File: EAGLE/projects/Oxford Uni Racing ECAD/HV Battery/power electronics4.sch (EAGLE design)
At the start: 57 parts, among them IC1 4043N, IC2 4001N, IC3 LM555CN, IC4 4071N, IC5 4081N, IC6 4011N, IC7 4011N, K1 T9AS1D12-48=T9A, K2 T9AS5D12-12=T9A, K4 T9AS1D12-48=T9A, K5 T9AS1D12-48=T9A, Q1 BS170, Q2 BS170, Q3 BS170

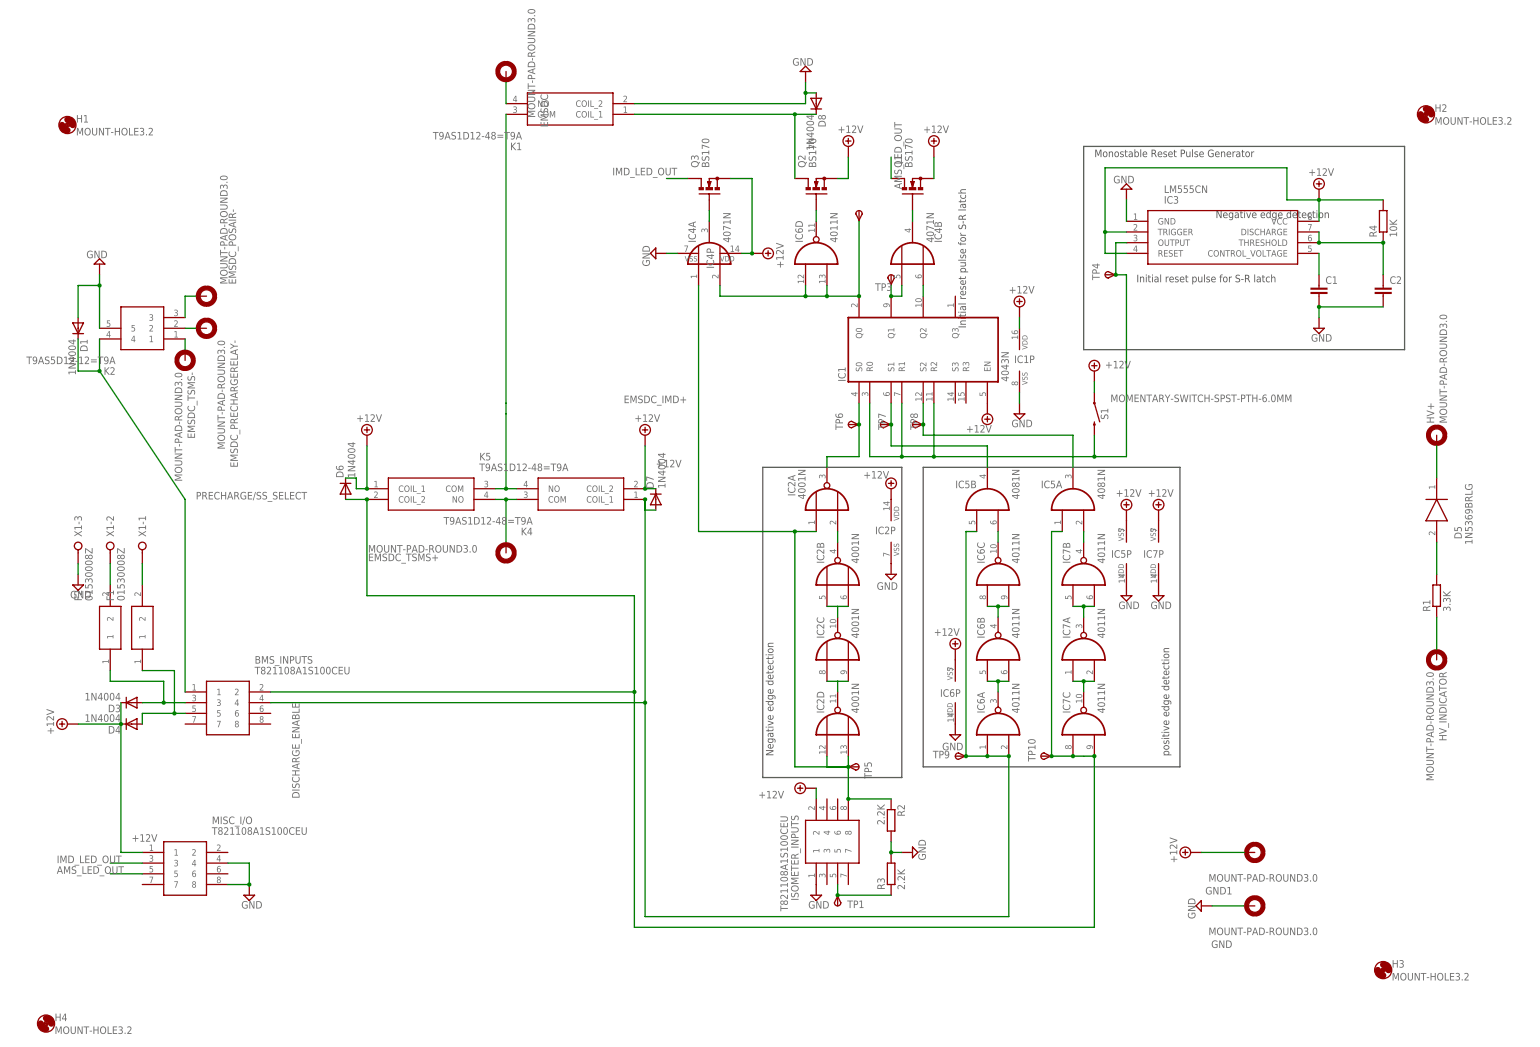
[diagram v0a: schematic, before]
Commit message: Modifications suggested by Dan after first review
Signed-off-by: Jack Bruford <jack.bruford41@gmail.com>
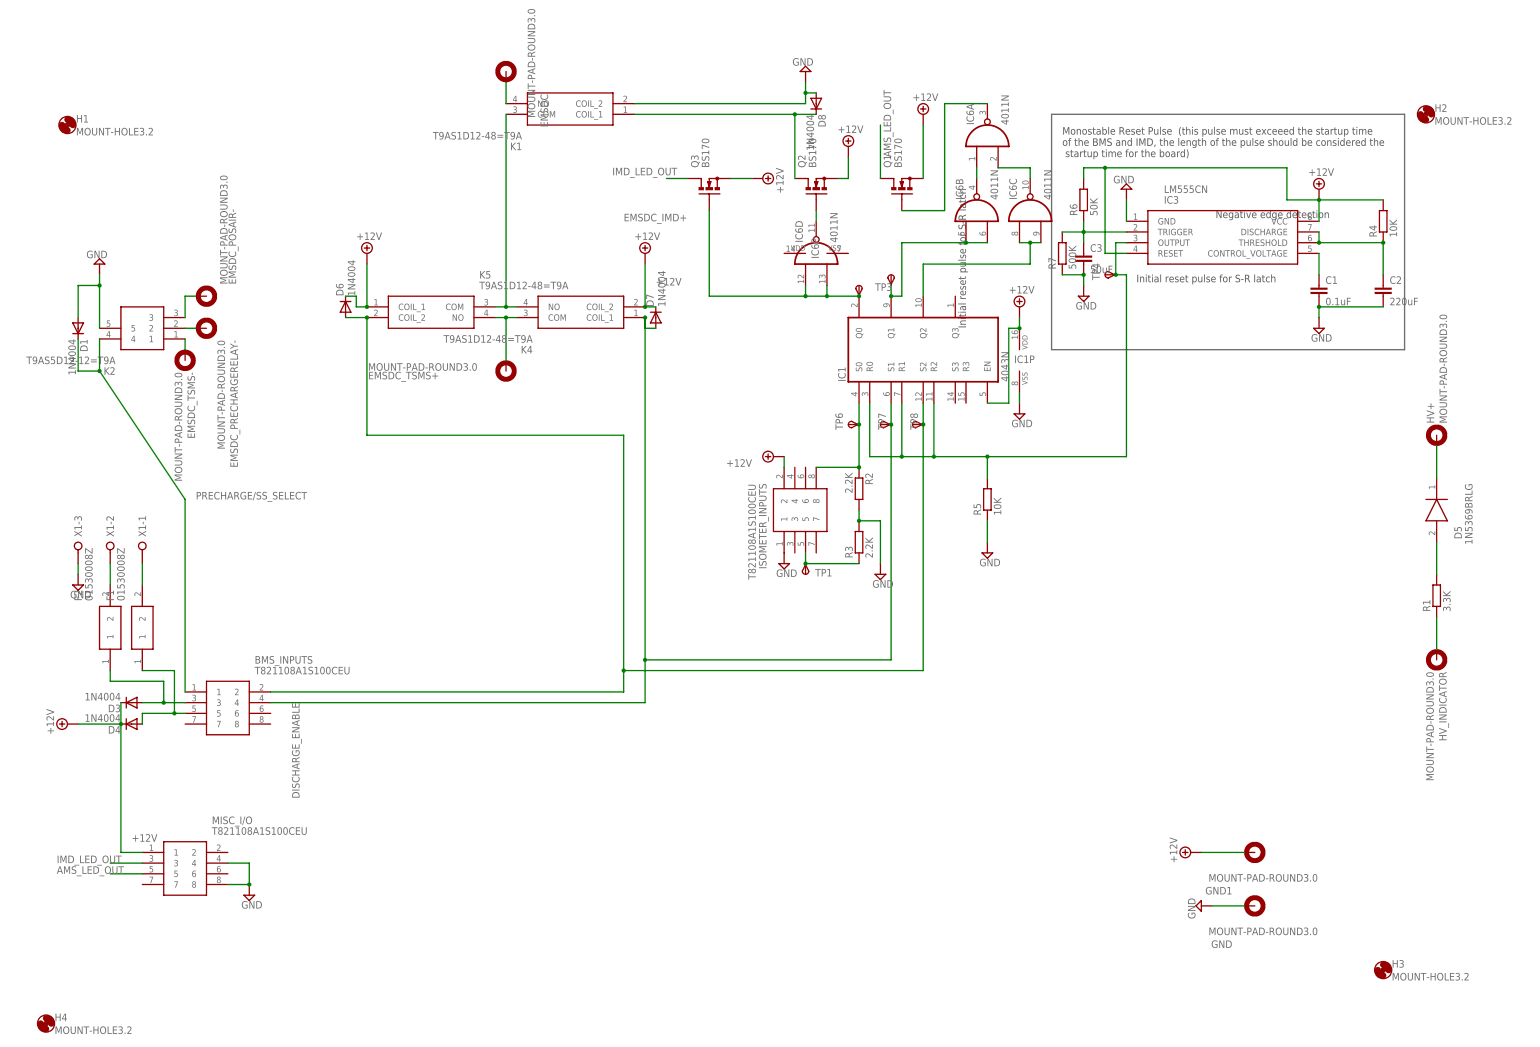
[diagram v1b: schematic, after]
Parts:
- removed IC2: 4001N, 40xx:4001N
- removed IC4: 4071N, 40xx:4071N
- removed IC5: 4081N, 40xx:4081N
- removed IC7: 4011N, 40xx:4011N
- removed S1: MOMENTARY-SWITCH-SPST-PTH-6.0MM, SparkFun-Switches:MOMENTARY-SWITCH-SPST-PTH-6.0MM
- removed TP10, TP5, TP9: TPSPAD1-17, testpad:TPSPAD1-17
- added C3: 50uF, rcl:C-EU050-024X044
- added R5: 10K, rcl:R-EU_0207/15
- added R6: 50K, rcl:R-EU_0207/15
- added R7: 500K, rcl:R-EU_0207/15
- C1: value (none) -> 0.1uF
- C2: value (none) -> 220uF
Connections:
- removed net N$23: IC1A.S1, IC5B.O, TP7.PP
- removed net N$24: IC6A.O, IC6B.I0, IC6B.I1
- removed net N$25: IC6B.O, IC6C.I0, IC6C.I1
- removed net N$26: IC5B.I1, IC6C.O
- removed net N$27: IC1A.S2, IC5A.O, TP8.PP
- removed net N$28: IC5A.I1, IC7B.O
- removed net N$29: IC1A.Q2, IC4B.I1
- removed net N$30: IC7A.O, IC7B.I0, IC7B.I1
- removed net N$32: IC7A.I0, IC7A.I1, IC7C.O
- removed net N$34: IC4B.O, Q1.G
- removed net N$36: IC5A.I0, IC7C.I0, TP10.PP
- net +12V: now also R6.2; no longer IC2P.VDD, IC3.TRIGGER, IC4P.VDD, IC5P.VSS, IC6P.VSS, IC7P.VSS, S1.1
- net CHG_SAFE: now also IC1A.S2, TP8.PP; no longer IC7C.I1
- net DISCHARGE_ENABLE: now also IC1A.S1, TP7.PP; no longer IC5B.I0, IC6A.I0, IC6A.I1, TP9.PP
- net GND: now also C3.2, R5.1, R7.1; no longer IC2P.VSS, IC4P.VSS, IC5P.VDD, IC6P.VDD, IC7P.VDD
- net N$11: now also IC1A.R0, IC1A.R1, IC1A.R2, IC3.OUTPUT, R5.2, TP4.PP; no longer IC2A.I0, IC2D.I0, IC2D.I1, IC4A.I0, ISOMETER_INPUTS.8, R2.1, TP5.PP
- net N$12: now also IC1A.Q1, IC6B.I0, IC6B.I1, TP3.PP; no longer IC2C.I0, IC2C.I1, IC2D.O
- net N$13: now also IC1A.Q2, IC6C.I0, IC6C.I1; no longer IC2B.I0, IC2B.I1, IC2C.O
- net N$14: now also IC6A.I0, IC6B.O; no longer IC2A.I1, IC2B.O
- net N$17: now also ISOMETER_INPUTS.8, R2.1; no longer IC2A.O
- net N$20: now also IC6A.I1, IC6C.O; no longer IC1A.R0, IC1A.R1, IC1A.R2, IC3.OUTPUT, S1.2, TP4.PP
- net N$21: now also IC6A.O, Q1.G; no longer IC1A.Q0, IC4A.I1, IC6D.I0, IC6D.I1, TP2.PP
- net N$22: now also C3.1, IC3.TRIGGER, R6.1, R7.2; no longer IC1A.Q1, IC4B.I0, TP3.PP
- net N$35: now also IC1A.Q0, IC6D.I0, IC6D.I1, TP2.PP; no longer IC4A.O
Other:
- note added: "Monostable Reset Pulse (this pulse must exceeed the startup time of the BMS and IMD, the length of the pulse should be considered the startup time for the board)"
- note removed: "Monostable Reset Pulse Generator"
- note removed: "positive edge detection"
- moved on the sheet: D6, D7, EMSDC_TSMS+, IC6A, IC6B, IC6C, IC6P, ISOMETER_INPUTS, K4, K5, Q1, R2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
